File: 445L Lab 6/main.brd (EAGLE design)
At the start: 38.1 x 63.5 mm, 45 parts, among them IC1 LM2937, IC2 LM4041CILPRLP, Q1 16MHz, U1 TM4C1233H6PM, U2 TPA731D, U3 TLV5616

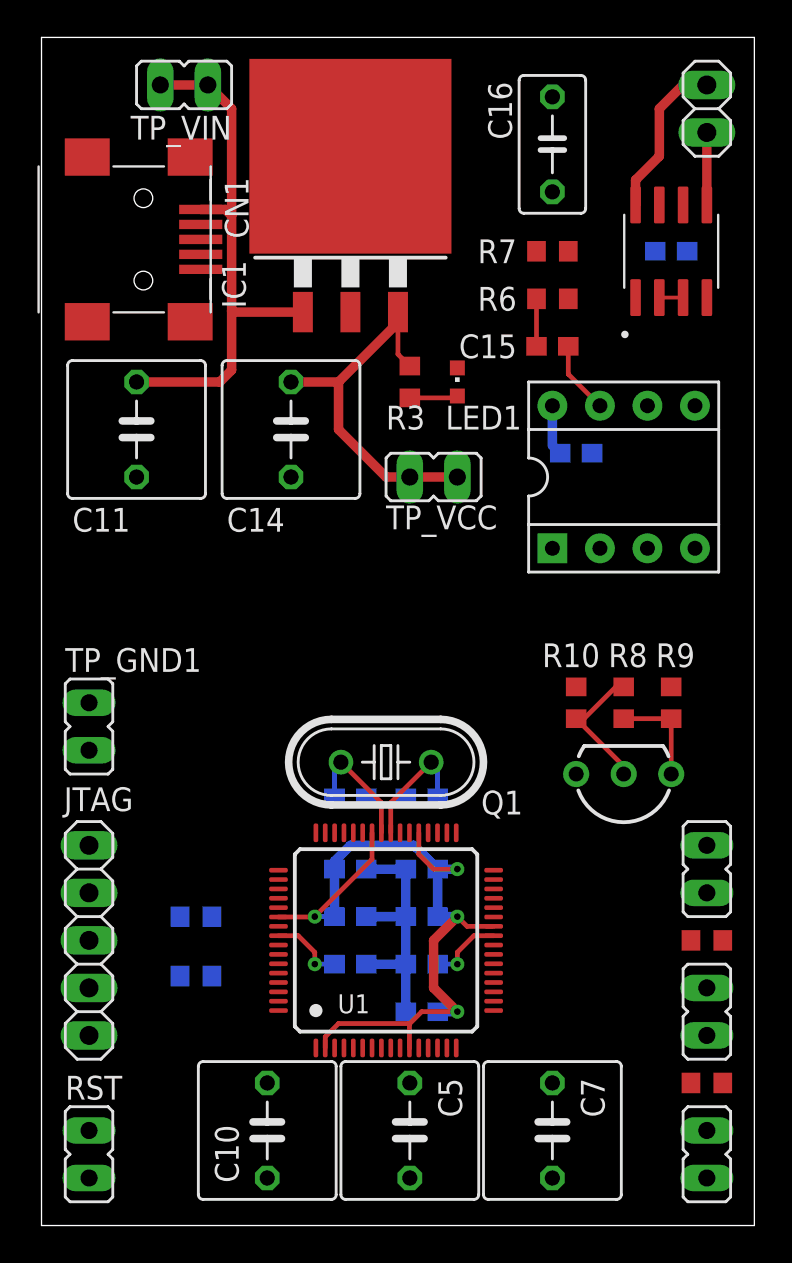
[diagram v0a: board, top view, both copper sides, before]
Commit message: Finished layout
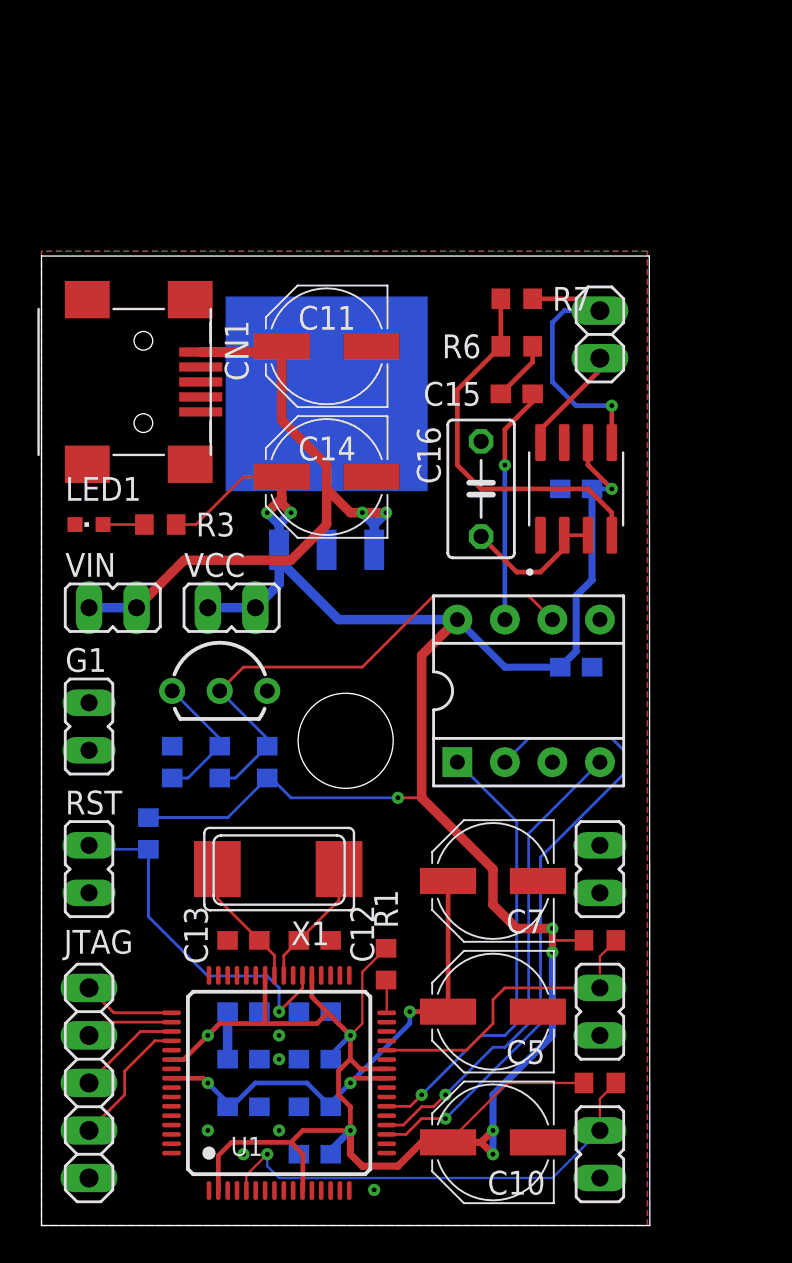
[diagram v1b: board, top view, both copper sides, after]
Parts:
- removed Q1: 16MHz, adafruit:HC49U-V
- removed TP_GND2, TP_VCC, TP_VIN: (no value), jumper:JP1
- added G2, VCC, VIN: (no value), jumper:JP1
- added X1: 16MHz, adafruit:NX8045
- C10, C11, C14, C5, C7: device rcl:C050-075X075 -> resistor:PANASONIC_D
- moved R9 26.9 mm to (6.99, 24.8), flipped to the bottom
- moved IC2 22.0 mm to (9.53, 28.6), turned to 0 degrees
- moved R8 21.8 mm to (9.53, 24.8), flipped to the bottom, turned to 90 degrees
- moved LED1 21.1 mm to (2.54, 37.5), turned to 90 degrees
- moved C16 18.8 mm to (23.5, 39.4)
- moved R10 16.8 mm to (12.1, 24.8), flipped to the bottom, turned to 270 degrees
- moved R3 15.4 mm to (6.35, 37.5), turned to 0 degrees
- moved RST 15.2 mm to (2.54, 19.1)
- moved C7 13.7 mm to (24.1, 18.4), turned to 180 degrees
- moved C18 13.7 mm to (28.6, 39.4)
- moved U2 13.7 mm to (28.6, 39.4)
- moved SPK 13.4 mm to (29.8, 47.6), turned to 270 degrees
- moved IC1 12.8 mm to (15.2, 41.9), flipped to the bottom
- moved U3 12.5 mm to (26.0, 28.6)
- moved C10 12.1 mm to (24.1, 4.45), turned to 180 degrees
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- renumbered TP_GND1 to G1
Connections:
- net 5V_IN: now also C11.+, VIN.1, VIN.2; no longer C11.1, TP_VIN.1, TP_VIN.2
- net GND: now also C10.-, C11.-, C14.-, C5.-, C7.-, G2.1, G2.2; no longer C10.2, C11.2, C14.2, C5.2, C7.2, TP_GND2.1, TP_GND2.2
- net OSC0: now also X1.P$2; no longer Q1.1
- net OSC1: now also X1.P$1; no longer Q1.2
- net VCC: now also C10.+, C14.+, VCC.1, VCC.2; no longer C10.1, C14.1, TP_VCC.1, TP_VCC.2
- net VDDC: now also C5.+, C7.+; no longer C5.1, C7.1
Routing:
- net VCC: track 68.5 -> 174.1 mm, vias 4 -> 11
- net SCLK: track 0.00 -> 34.3 mm, vias 0 -> 1
- net FSS: track 0.00 -> 25.4 mm, vias 0 -> 1
- net PF4: track 0.00 -> 25.0 mm, vias 0 -> 1
- net MOSI: track 0.00 -> 24.1 mm, vias 0 -> 1
- net VREF: track 7.26 -> 27.7 mm
- net AMP_IN-: track 0.00 -> 20.4 mm
- net VDDC: track 7.99 -> 28.2 mm, vias 2 -> 3
- net RST: track 0.00 -> 19.1 mm, vias 0 -> 1
- net PF0: track 0.00 -> 16.4 mm
- net GND: track 13.9 -> 0.00 mm, vias 0 -> 6
- net VO+: track 3.88 -> 15.5 mm, vias 0 -> 1
- net VDAC: track 3.88 -> 12.7 mm, vias 0 -> 1
- net 5V_IN: track 29.3 -> 37.7 mm, vias 0 -> 2
- net TCK: track 0.00 -> 7.14 mm
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- added copper zone on layer 1, net GND
- added copper zone on layer 16, net GND
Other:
- board size 38.1 x 63.5 mm -> 32.5 x 51.8 mm
